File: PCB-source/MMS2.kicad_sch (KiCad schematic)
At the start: 4 parts

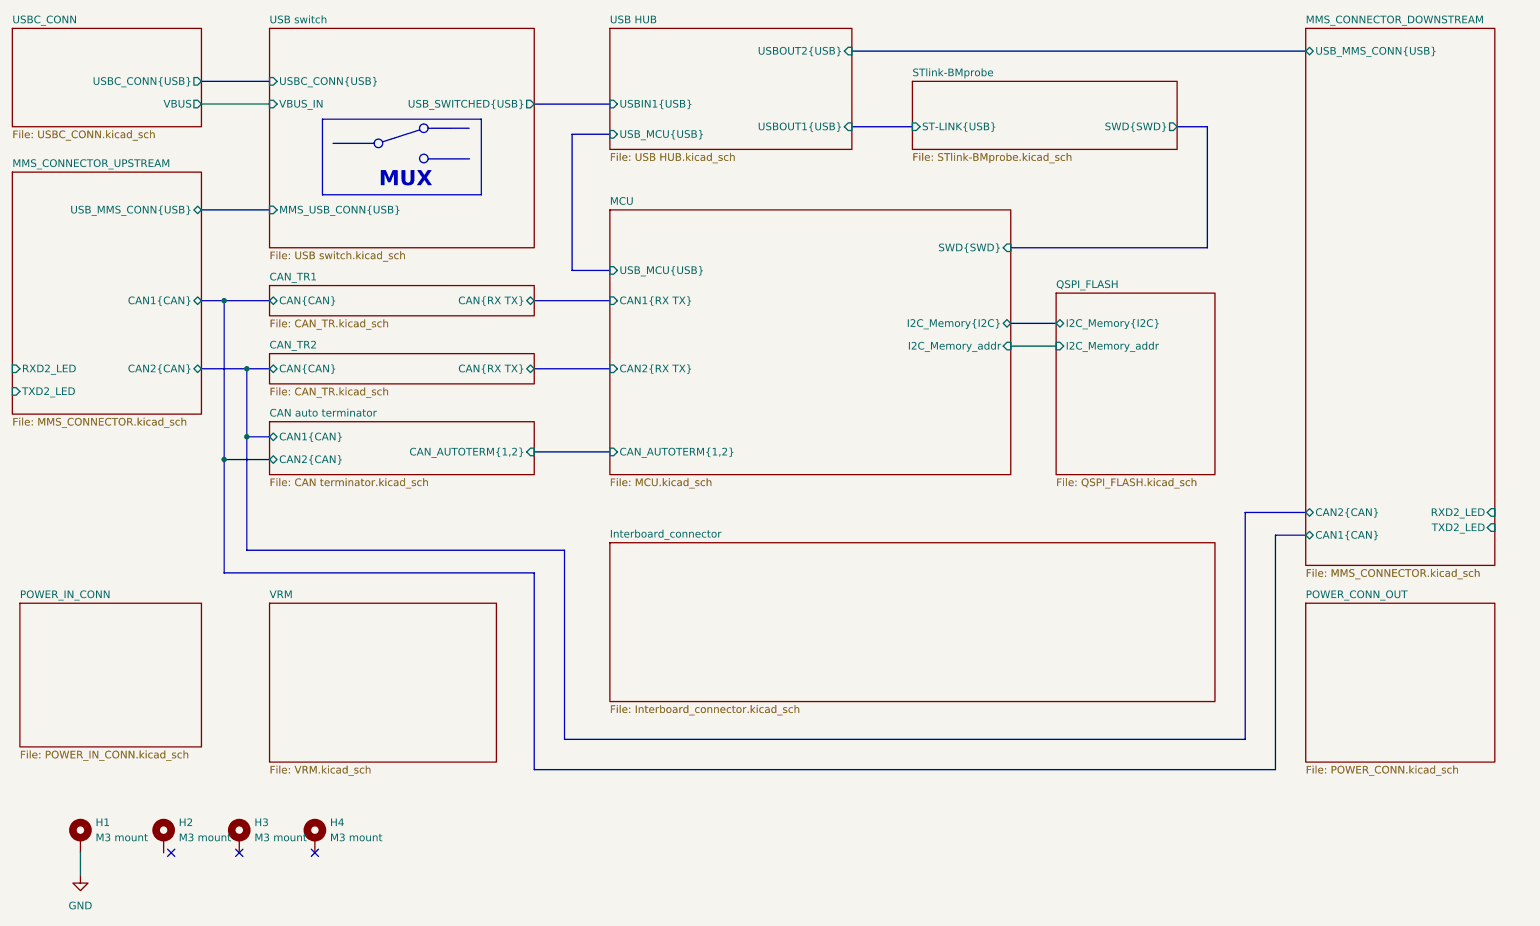
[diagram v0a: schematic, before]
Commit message: ch32
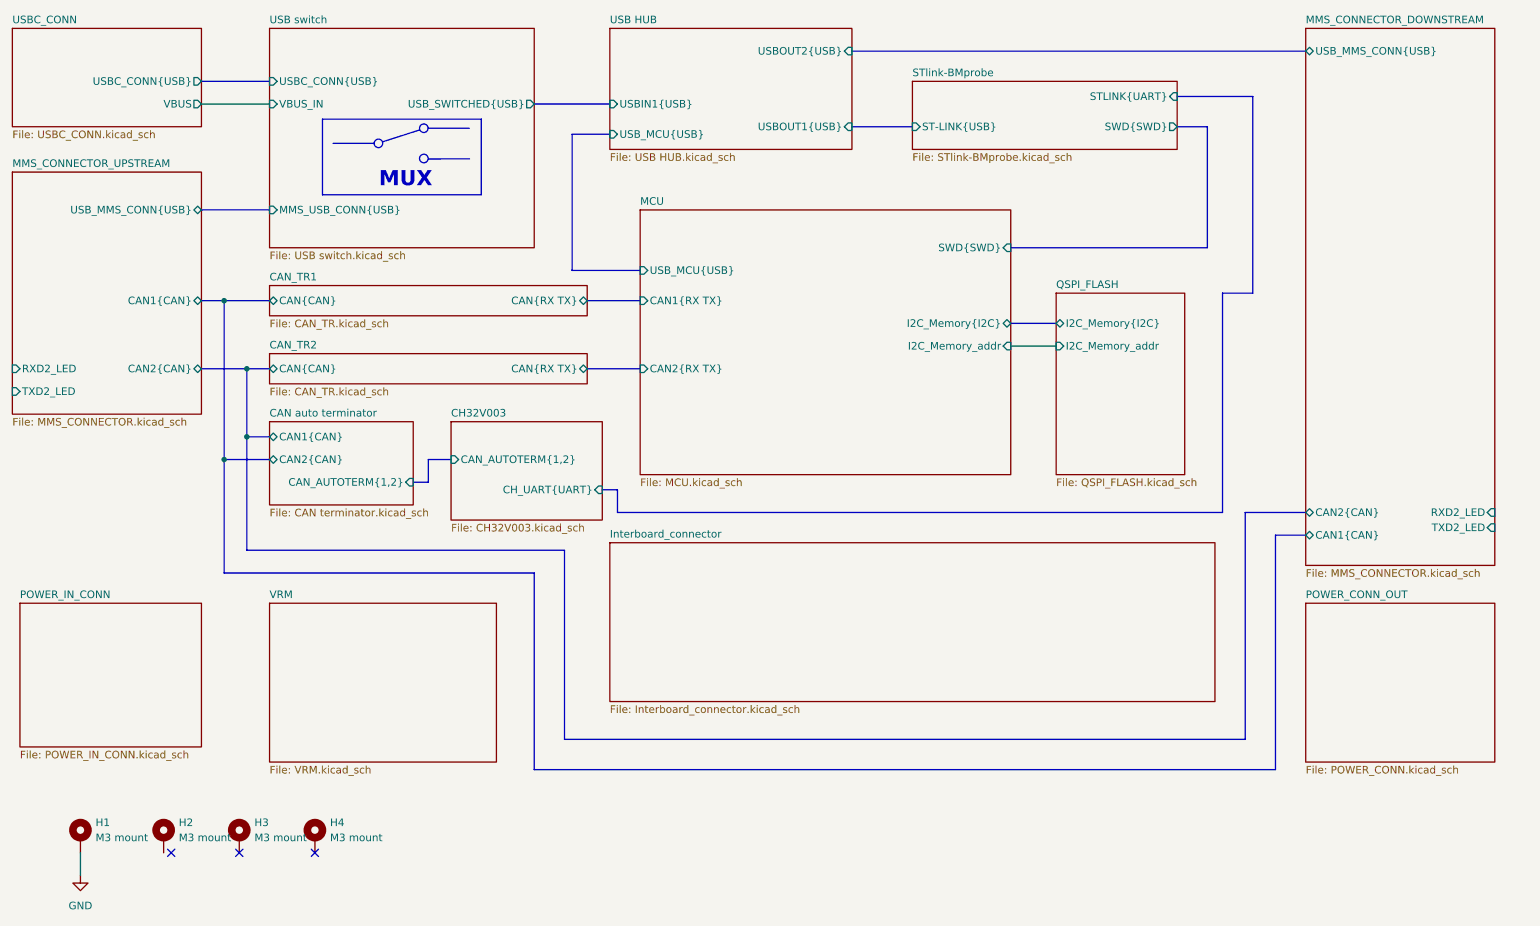
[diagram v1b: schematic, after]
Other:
- added sheet CH32V003 (CH32V003.kicad_sch)
- sheet MCU ports: added none; removed CAN_AUTOTERM{1,2}
- sheet STlink-BMprobe ports: added STLINK{UART}; removed none
